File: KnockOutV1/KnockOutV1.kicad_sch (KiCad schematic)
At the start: 1 part, among them U1 STM32F103C8T6

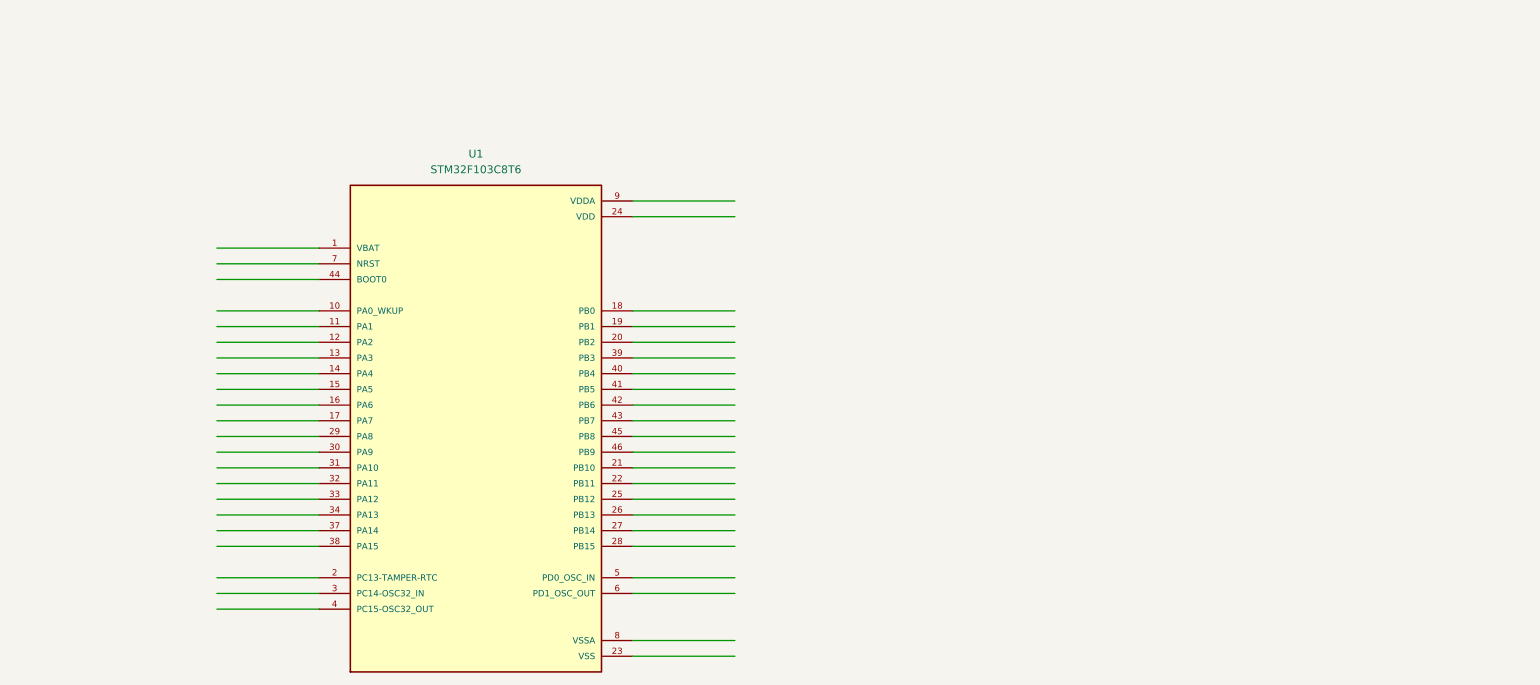
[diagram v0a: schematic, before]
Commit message: Added to Schematics
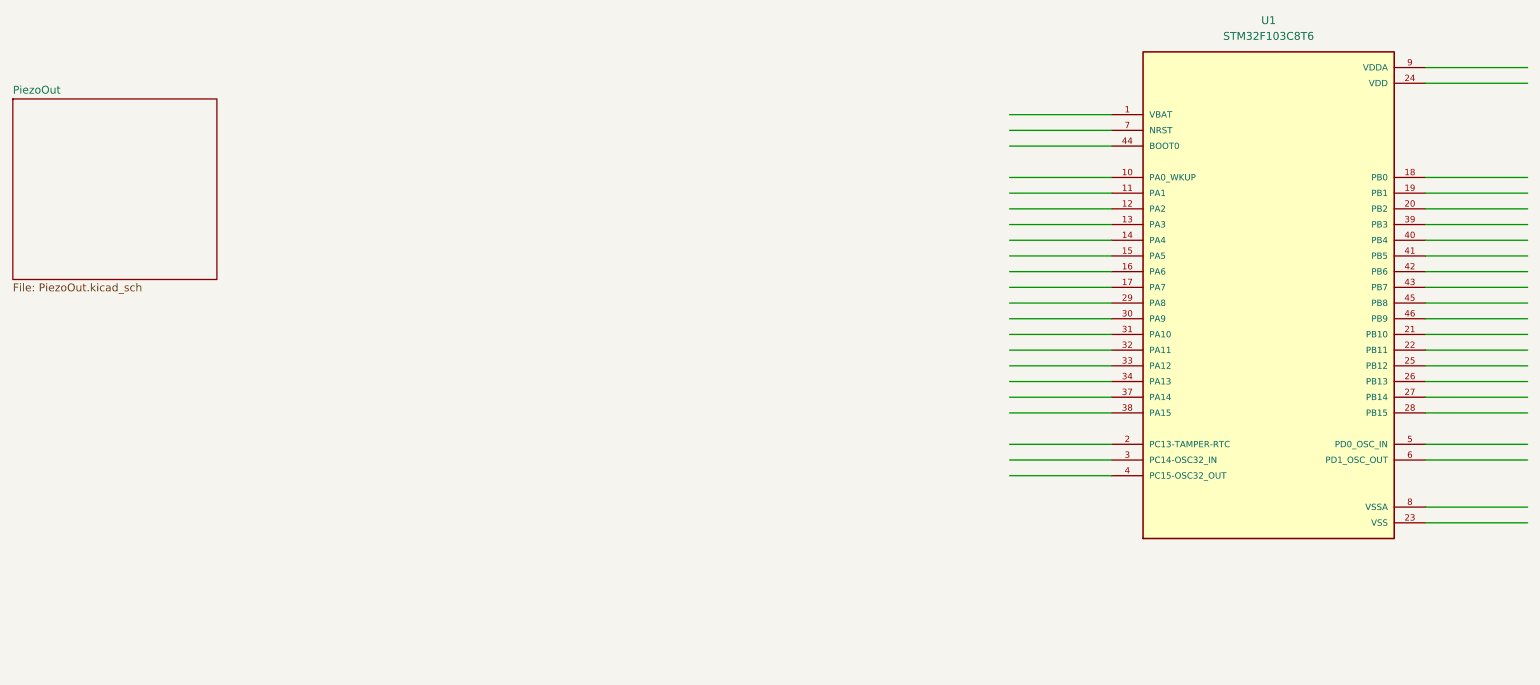
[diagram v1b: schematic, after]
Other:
- added sheet PiezoOut (PiezoOut.kicad_sch)
- moved on the sheet: U1
